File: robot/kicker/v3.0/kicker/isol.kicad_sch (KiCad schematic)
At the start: 11 parts, among them J4 Conn_01x10, U6 ISO6720-Q1, U7 ISO6720-Q1, U8 ISO6721-Q1

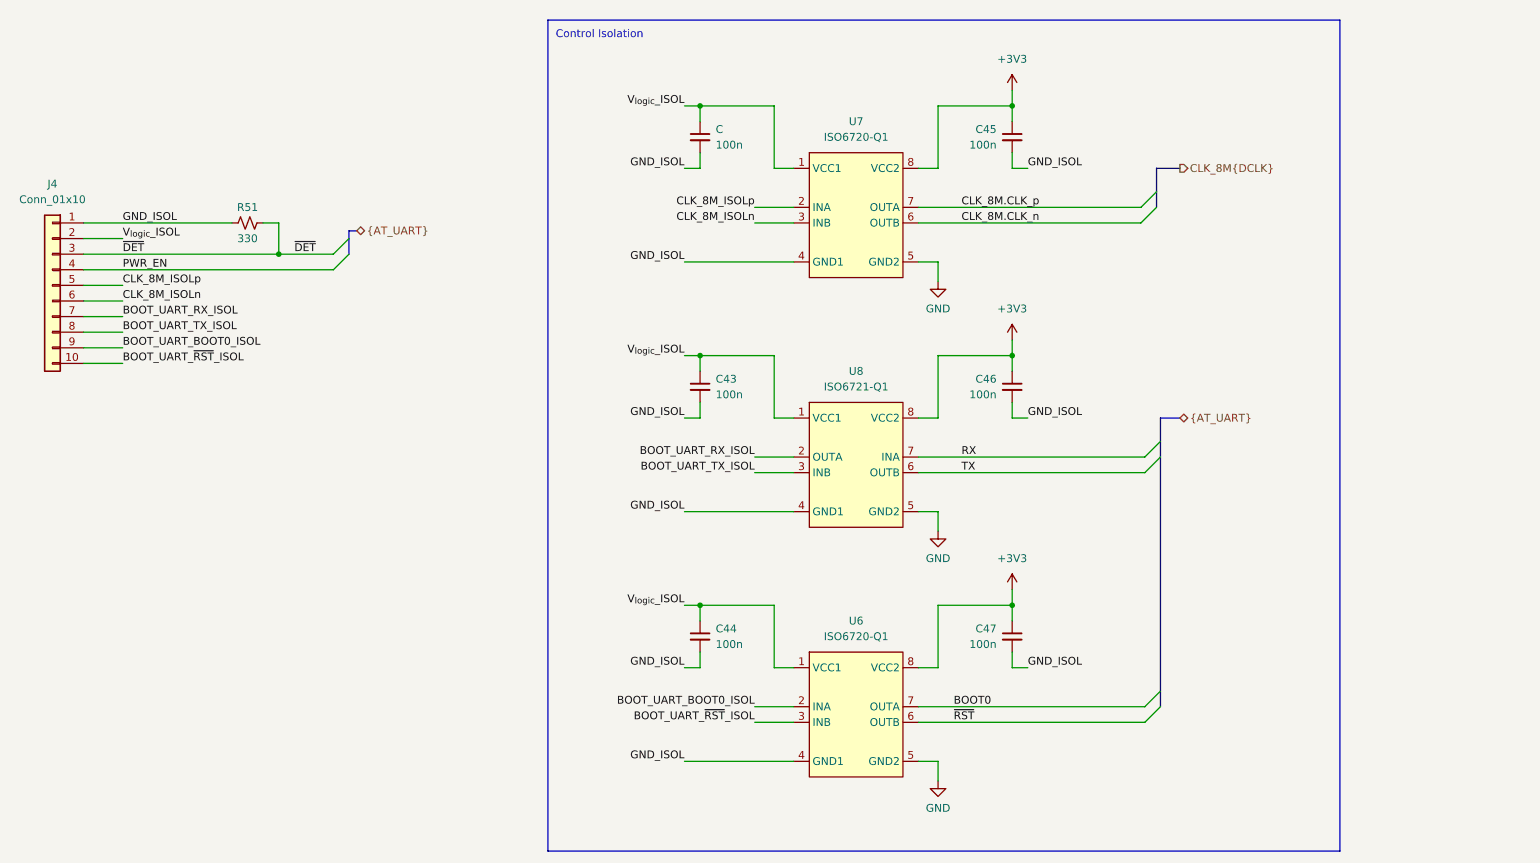
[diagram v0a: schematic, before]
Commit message: lots of ERC work
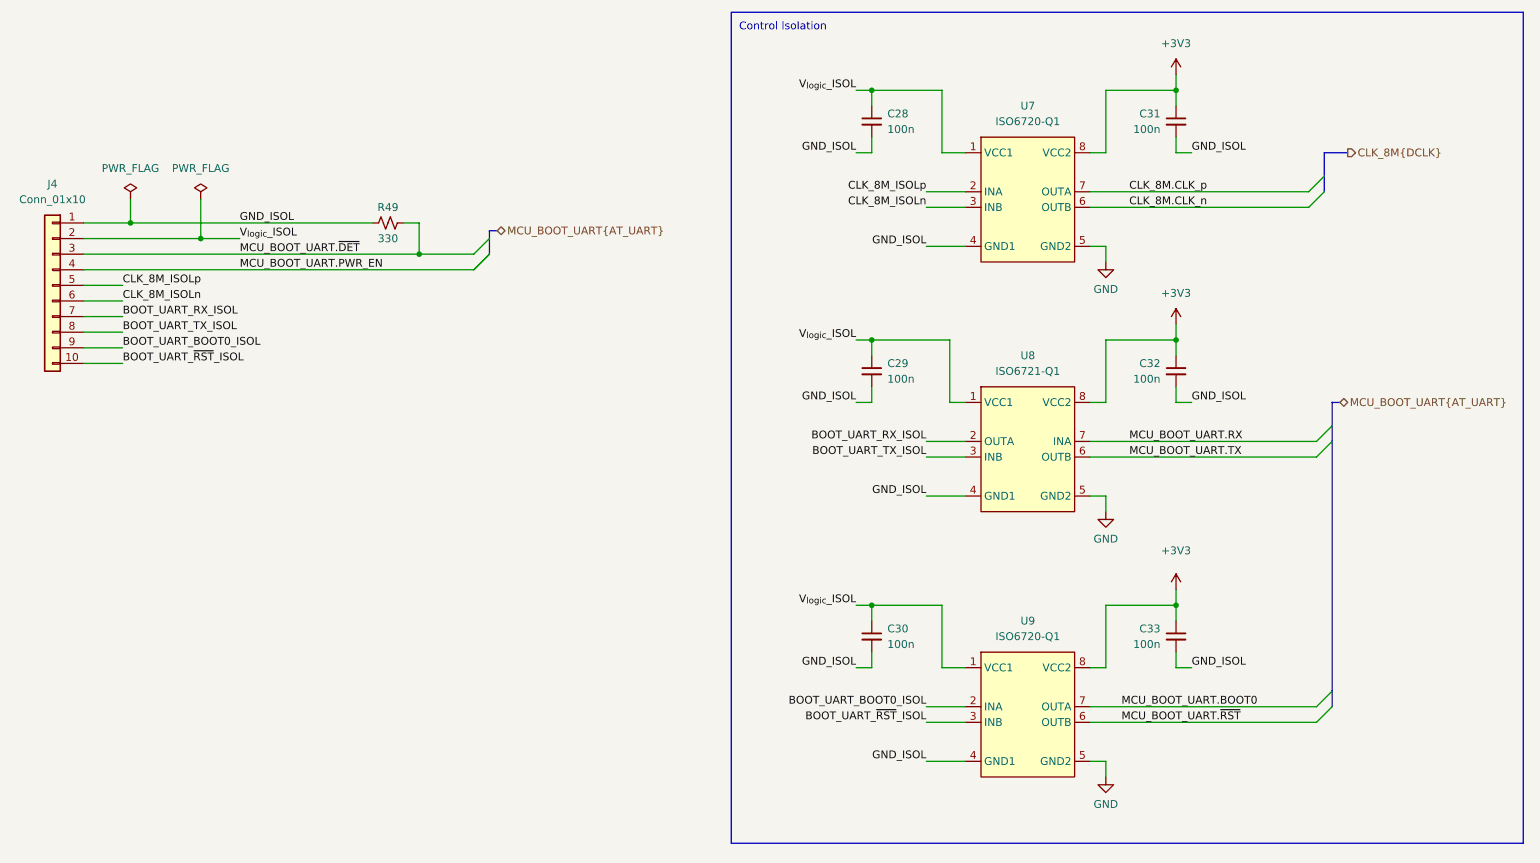
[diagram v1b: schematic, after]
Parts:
- renumbered C to C28, C43 to C29, C44 to C30, C45 to C31, C46 to C32, C47 to C33, R51 to R49, U6 to U9
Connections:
- net BOOT0 renamed MCU_BOOT_UART.BOOT0
- net PWR_EN renamed MCU_BOOT_UART.PWR_EN
- net RX renamed MCU_BOOT_UART.RX
- net TX renamed MCU_BOOT_UART.TX
- net ~{DET} renamed MCU_BOOT_UART.~{DET}
- net ~{RST} renamed MCU_BOOT_UART.~{RST}
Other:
- moved on the sheet: C28, C29, C30, C31, C32, C33, R49, U7, U8, U9
